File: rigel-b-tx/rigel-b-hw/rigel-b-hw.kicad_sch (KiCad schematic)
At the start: 46 parts, among them IC1 BALFHB-WL-02D3, J1 Conn_01x03_Pin, J2 436500200, J3 Conn_01x03_Pin, U1 STM32WLE5C8Ux, U2 TPS629206DRLR, U3 CH340X, U4 TYPE-C_16PIN_2MD(073), U5 X1G004131004200, U6 KH-SMA-K513-G, U7 MSK12C02-HB

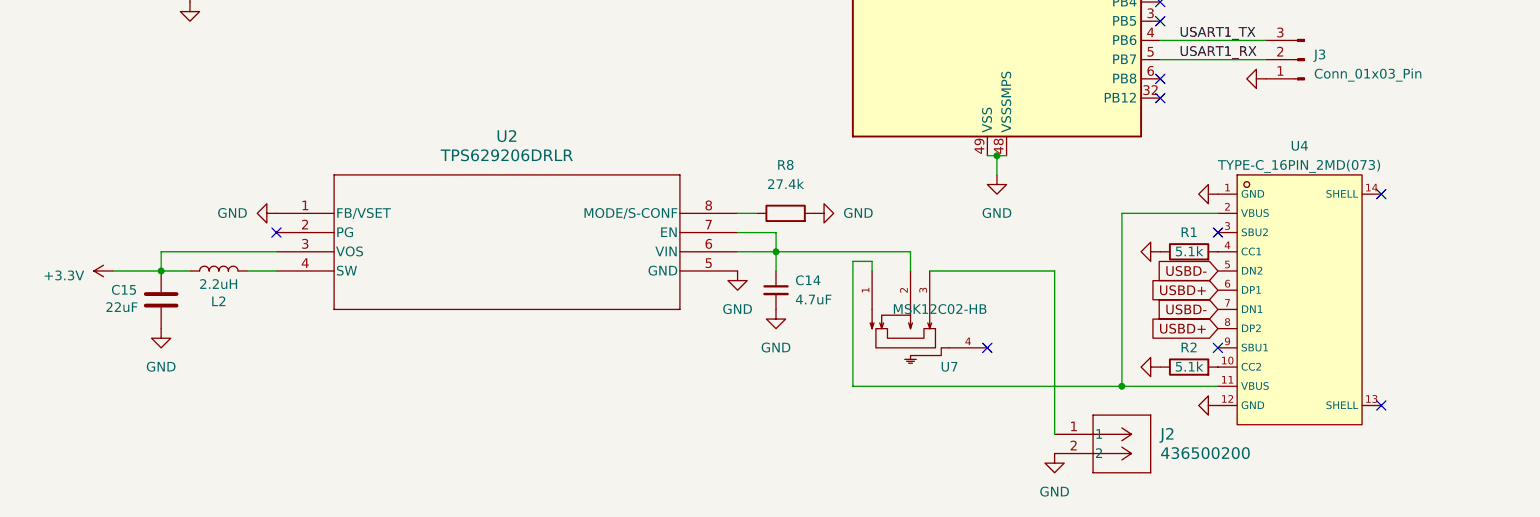
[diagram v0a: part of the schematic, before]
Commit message: Diodes
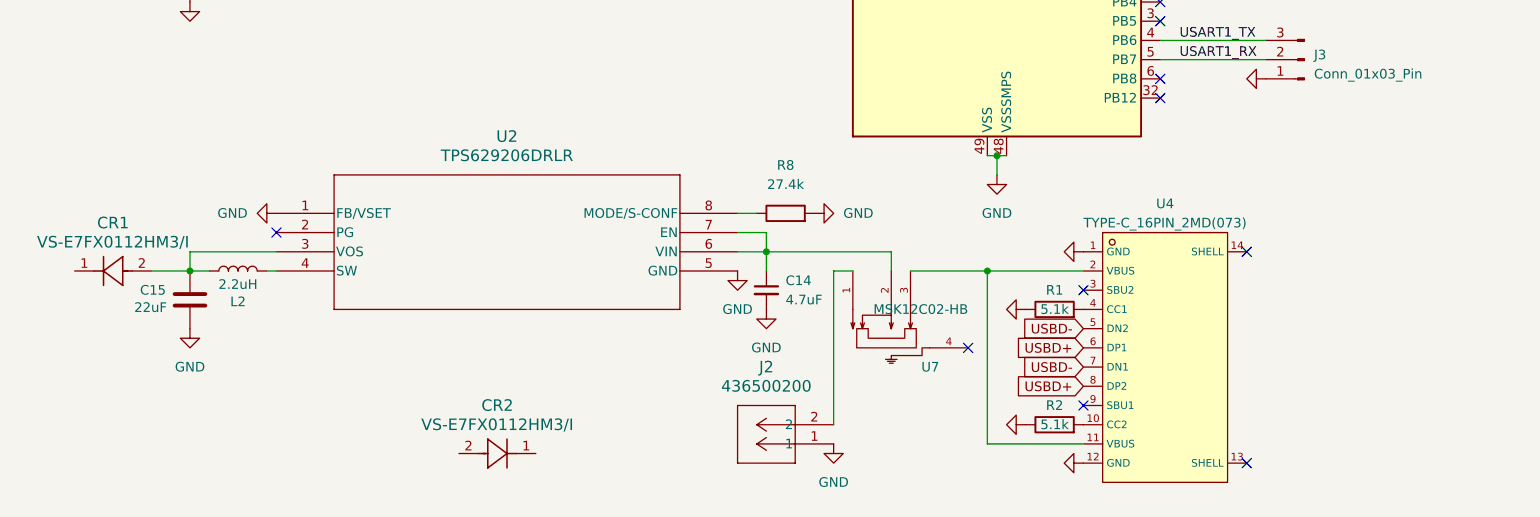
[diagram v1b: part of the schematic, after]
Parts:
- added CR1, CR2: VS-E7FX0112HM3/I, CR_SMF_DO-219AB_VIS, symbol 2024-11-05_21-21-38:VS-E7FX0112HM3_I
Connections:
- net +3.3V: no longer C15.2, L2.1, U2.3 (VOS)
- net GND: now also J2.1; no longer J2.2
- net at U4.11 (VBUS), U4.2 (VBUS): now also U7.3; no longer U7.1
- new net: C15.2, CR1.2, L2.1, U2.3 (VOS)
- new net: J2.2, U7.1
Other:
- moved on the sheet: C14, C15, J2, L2, R1, R2, U4, U7
